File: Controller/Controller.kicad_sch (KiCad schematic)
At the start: 33 parts, among them J1 USB_B, SW2 SW_Push, SW3 SW_Push, SW4 SW_Push, SW5 SW_Push, SW6 SW_Push, SW7 SW_Push, SW8 SW_Push, SW9 SW_Push

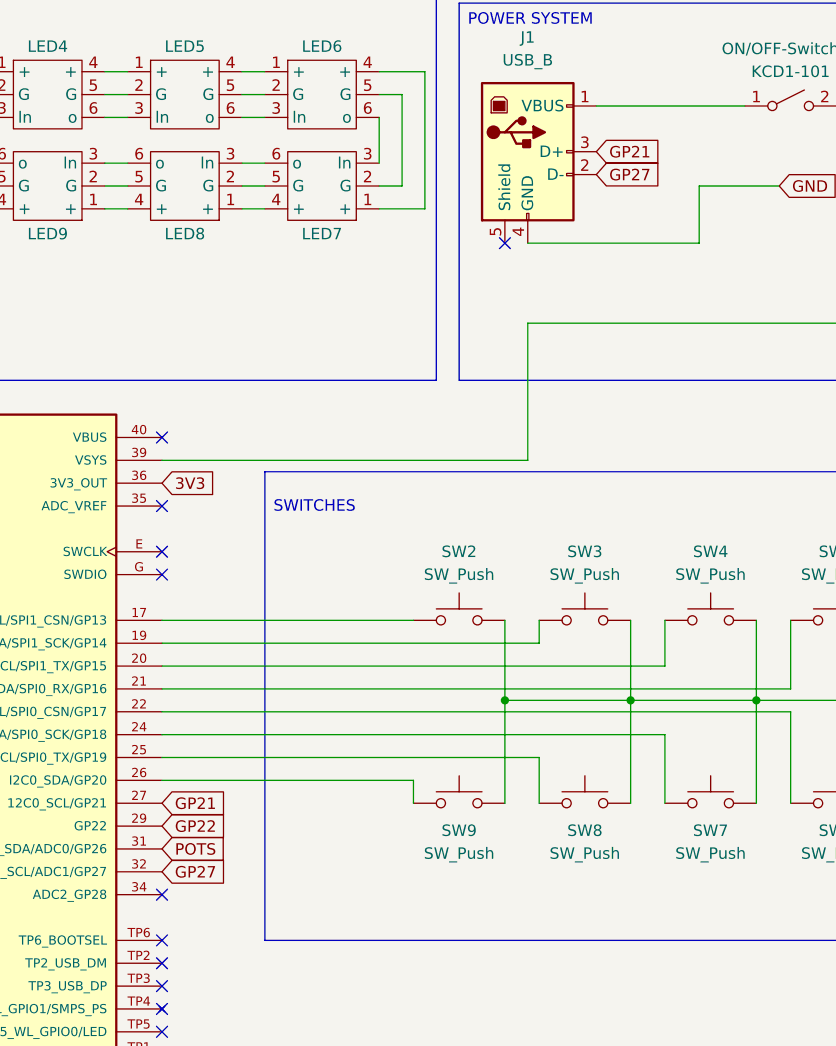
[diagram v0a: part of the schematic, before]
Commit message: Fix i2c
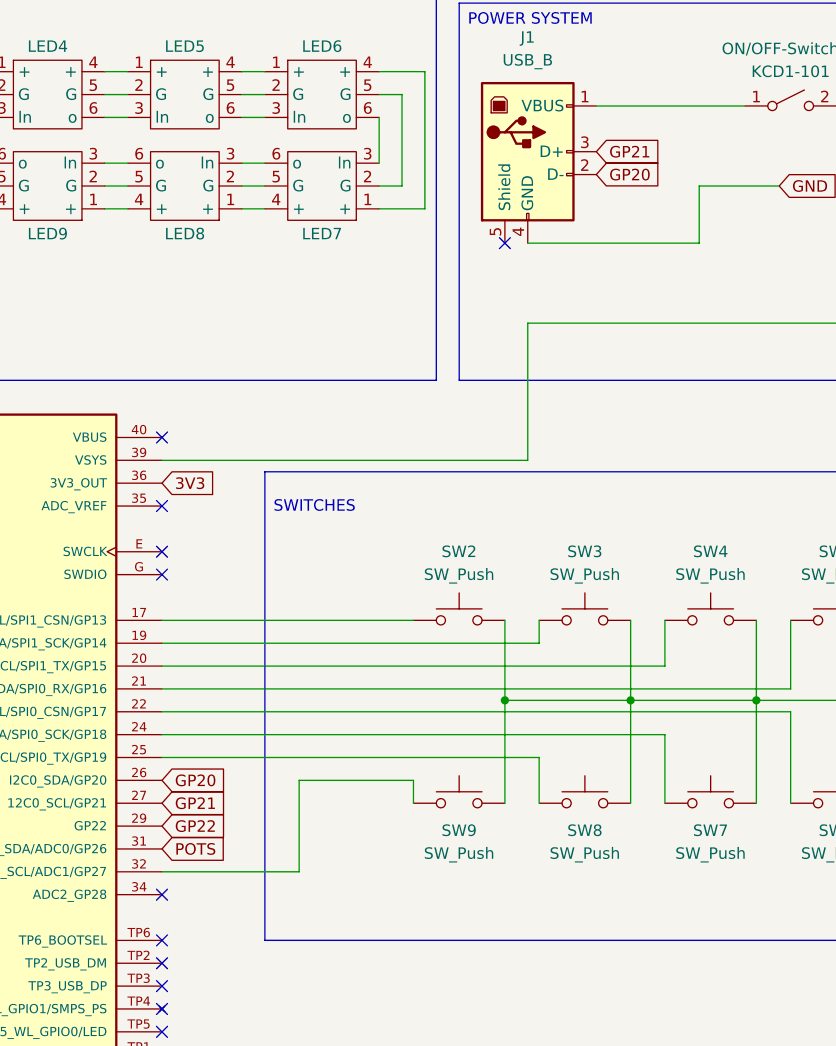
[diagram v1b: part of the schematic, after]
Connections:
- net at SW9.1: now also PICO-1.32 (I2C1_SCL/ADC1/GP27); no longer PICO-1.26 (I2C0_SDA/GP20)
- net GP27 renamed GP20
- net GP20: now also PICO-1.26 (I2C0_SDA/GP20); no longer PICO-1.32 (I2C1_SCL/ADC1/GP27)

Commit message: Fix mistakes
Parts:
- NFC-1: footprint Connector_PinHeader_2.54mm:PinHeader_1x07_P2.54mm_Vertical -> Connector_PinHeader_2.54mm:PinHeader_1x08_P2.54mm_Vertical
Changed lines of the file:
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@@
 			)
 		)
-		(property "Footprint" "Connector_PinHeader_2.54mm:PinHeader_1x07_P2.54mm_Vertical"
+		(property "Footprint" "Connector_PinHeader_2.54mm:PinHeader_1x08_P2.54mm_Vertical"
 			(at 38.1 76.2 0)
 			(effects
